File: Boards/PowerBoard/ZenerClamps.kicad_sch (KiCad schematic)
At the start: 24 parts

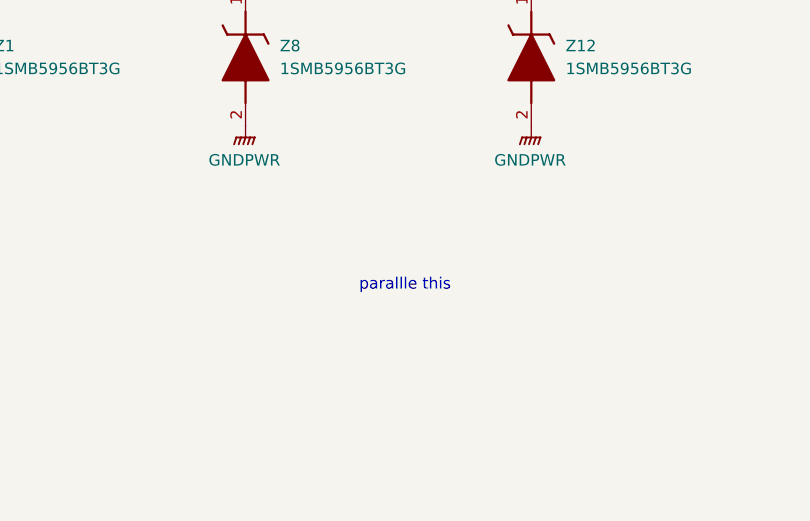
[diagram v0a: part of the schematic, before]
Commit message: Update Layouts
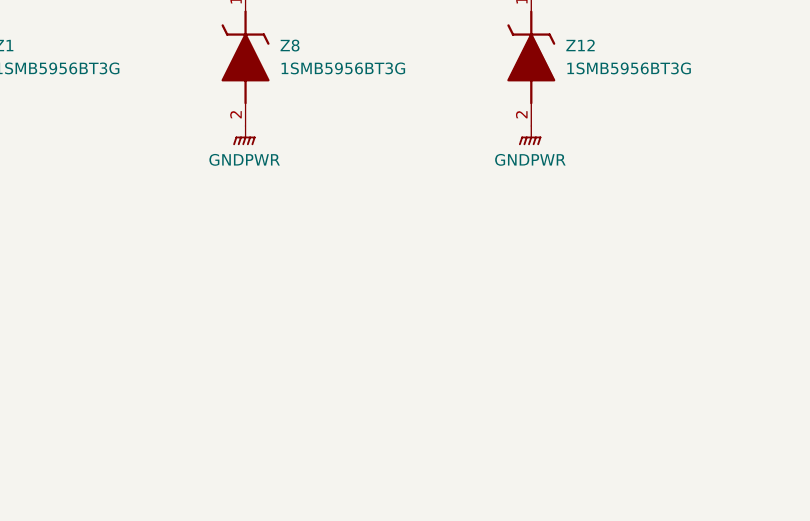
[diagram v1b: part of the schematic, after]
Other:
- note removed: "parallle this"
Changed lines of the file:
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@@
 	(generator_version "9.0")
 	(paper "A4")
-	(text "parallle this\n"
-		(exclude_from_sim no)
-		(at 74.8662 104.0919 0)
-		(effects
-			(font
-				(size 1.27 1.27)
-			)
-		)
-	)
 	(global_label "PHASE_U"
 		(shape input)
